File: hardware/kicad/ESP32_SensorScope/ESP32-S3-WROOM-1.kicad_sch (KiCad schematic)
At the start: 17 parts, among them J9 USB_C_Receptacle_USB2.0_16P, SW2 Reset, SW3 Boot, U15 LM1117MP-3.3, U2 ESP32-S3-WROOM-1

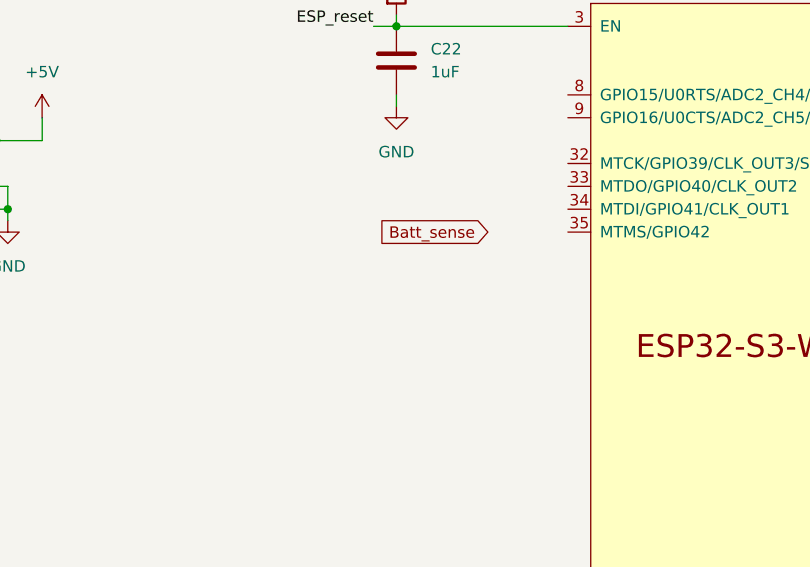
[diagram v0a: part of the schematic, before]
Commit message: something probobly
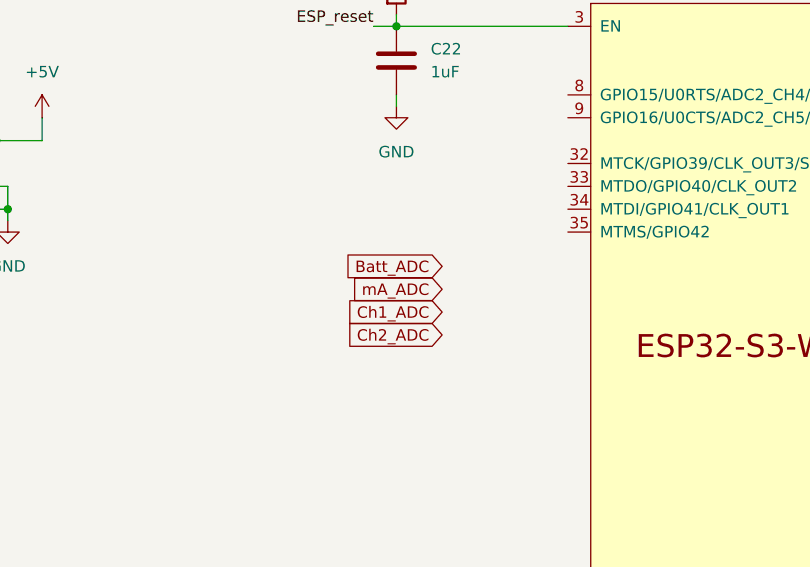
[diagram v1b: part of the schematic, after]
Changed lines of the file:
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@@
 		)
 	)
-	(global_label "Batt_sense"
+	(global_label "Ch2_ADC"
 		(shape input)
-		(at 137.16 59.69 180)
+		(at 132.08 71.12 180)
 		(fields_autoplaced yes)
 		(effects
@@
 		)
 		(property "Intersheetrefs" "${INTERSHEET_REFS}"
-			(at 123.9544 59.69 0)
+			(at 120.8701 71.12 0)
+			(effects
+				(font
+					(size 1.27 1.27)
+				)
+				(justify right)
+				(hide yes)
+			)
+		)
+	)
+	(global_label "Batt_ADC"
+		(shape input)
+		(at 132.08 63.5 180)
+		(fields_autoplaced yes)
+		(effects
+			(font
+				(size 1.27 1.27)
+			)
+			(justify right)
+		)
+		(property "Intersheetrefs" "${INTERSHEET_REFS}"
+			(at 120.6282 63.5 0)
 			(effects
 				(font
@@
 				)
 				(justify left)
+				(hide yes)
+			)
+		)
+	)
+	(global_label "mA_ADC"
+		(shape input)
+		(at 132.08 66.04 180)
+		(fields_autoplaced yes)
+		(effects
+			(font
+				(size 1.27 1.27)
+			)
+			(justify right)
+		)
+		(property "Intersheetrefs" "${INTERSHEET_REFS}"
+			(at 121.7167 66.04 0)
+			(effects
+				(font
+					(size 1.27 1.27)
+				)
+				(justify right)
 				(hide yes)
 			)
@@
 			(effects
 				(font
+					(size 1.27 1.27)
+				)
+				(justify right)
+				(hide yes)
+			)
+		)
+	)
+	(global_label "Ch1_ADC"
+		(shape input)
+		(at 132.08 68.58 180)
+		(fields_autoplaced yes)
+		(effects
+			(font
+				(size 1.27 1.27)
+			)
+			(justify right)
+		)
+		(property "Intersheetrefs" "${INTERSHEET_REFS}"
+			(at 120.8701 68.58 0)
+			(effects
+				(font
